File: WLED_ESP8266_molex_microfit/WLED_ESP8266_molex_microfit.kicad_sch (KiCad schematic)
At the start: 65 parts, among them J1 Molex Micro-fit 2x1, J2 Molex Micro-fit 3x1, J3 Molex Micro-fit 2x1, J4 Molex Micro-fit 2x1, J5 USB_B_Micro, J6 Molex Micro-fit 2x1, J7 Molex Micro-fit 3x1, J8 Molex Micro-fit 3x1, Q1 AO3401A, Q2 AO3401A, U1 ESP-12F, U2 TPS54331DDAR, U3 TXS0102DCT, U4 TXS0102DCT, U6 ME6211A33M3G-N

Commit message: Issue 28.01.Yannik_part1
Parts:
- R1, R10, R12, R13, R14, R15, R16, R17: footprint Capacitor_SMD:C_0402_1005Metric_Pad0.74x0.62mm_HandSolder -> Resistor_SMD:R_0402_1005Metric_Pad0.72x0.64mm_HandSolder
- R18, R7, R8, R9: footprint Capacitor_SMD:C_0603_1608Metric_Pad1.08x0.95mm_HandSolder -> Resistor_SMD:R_0603_1608Metric_Pad0.98x0.95mm_HandSolder
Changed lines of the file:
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@@
     (property "Reference" "R12" (id 0) (at 46.99 83.82 90))
     (property "Value" "10k" (id 1) (at 50.8 87.63 90))
-    (property "Footprint" "Capacitor_SMD:C_0402_1005Metric_Pad0.74x0.62mm_HandSolder" (id 2) (at 50.038 87.63 90)
+    (property "Footprint" "Resistor_SMD:R_0402_1005Metric_Pad0.72x0.64mm_HandSolder" (id 2) (at 50.038 87.63 90)
       (effects (font (size 1.27 1.27)) hide)
     )
@@
     (property "Reference" "R8" (id 0) (at 259.08 39.37 90))
     (property "Value" "300" (id 1) (at 255.27 43.18 90))
-    (property "Footprint" "Capacitor_SMD:C_0603_1608Metric_Pad1.08x0.95mm_HandSolder" (id 2) (at 255.27 42.418 90)
+    (property "Footprint" "Resistor_SMD:R_0603_1608Metric_Pad0.98x0.95mm_HandSolder" (id 2) (at 255.27 42.418 90)
       (effects (font (size 1.27 1.27)) hide)
     )
@@
     (property "Reference" "R17" (id 0) (at 166.37 91.44 90))
     (property "Value" "10k" (id 1) (at 171.45 92.71 90))
-    (property "Footprint" "Capacitor_SMD:C_0402_1005Metric_Pad0.74x0.62mm_HandSolder" (id 2) (at 170.688 92.71 90)
+    (property "Footprint" "Resistor_SMD:R_0402_1005Metric_Pad0.72x0.64mm_HandSolder" (id 2) (at 170.688 92.71 90)
       (effects (font (size 1.27 1.27)) hide)
     )
@@
     (property "Reference" "R15" (id 0) (at 118.11 91.44 90))
     (property "Value" "10k" (id 1) (at 123.19 92.71 90))
-    (property "Footprint" "Capacitor_SMD:C_0402_1005Metric_Pad0.74x0.62mm_HandSolder" (id 2) (at 122.428 92.71 90)
+    (property "Footprint" "Resistor_SMD:R_0402_1005Metric_Pad0.72x0.64mm_HandSolder" (id 2) (at 122.428 92.71 90)
       (effects (font (size 1.27 1.27)) hide)
     )
@@
     (property "Reference" "R9" (id 0) (at 259.08 90.17 90))
     (property "Value" "300" (id 1) (at 255.27 93.98 90))
-    (property "Footprint" "Capacitor_SMD:C_0603_1608Metric_Pad1.08x0.95mm_HandSolder" (id 2) (at 255.27 93.218 90)
+    (property "Footprint" "Resistor_SMD:R_0603_1608Metric_Pad0.98x0.95mm_HandSolder" (id 2) (at 255.27 93.218 90)
       (effects (font (size 1.27 1.27)) hide)
     )
@@
     (property "Reference" "R14" (id 0) (at 62.23 83.82 90))
     (property "Value" "10k" (id 1) (at 66.04 87.63 90))
-    (property "Footprint" "Capacitor_SMD:C_0402_1005Metric_Pad0.74x0.62mm_HandSolder" (id 2) (at 65.278 87.63 90)
+    (property "Footprint" "Resistor_SMD:R_0402_1005Metric_Pad0.72x0.64mm_HandSolder" (id 2) (at 65.278 87.63 90)
       (effects (font (size 1.27 1.27)) hide)
     )
@@
     (property "Reference" "R7" (id 0) (at 259.08 34.29 90))
     (property "Value" "300" (id 1) (at 255.27 38.1 90))
-    (property "Footprint" "Capacitor_SMD:C_0603_1608Metric_Pad1.08x0.95mm_HandSolder" (id 2) (at 255.27 37.338 90)
+    (property "Footprint" "Resistor_SMD:R_0603_1608Metric_Pad0.98x0.95mm_HandSolder" (id 2) (at 255.27 37.338 90)
       (effects (font (size 1.27 1.27)) hide)
     )
@@
     (property "Reference" "R1" (id 0) (at 17.78 86.36 90))
     (property "Value" "10k" (id 1) (at 21.59 90.17 90))
-    (property "Footprint" "Capacitor_SMD:C_0402_1005Metric_Pad0.74x0.62mm_HandSolder" (id 2) (at 20.828 90.17 90)
+    (property "Footprint" "Resistor_SMD:R_0402_1005Metric_Pad0.72x0.64mm_HandSolder" (id 2) (at 20.828 90.17 90)
       (effects (font (size 1.27 1.27)) hide)
     )
@@
     (property "Reference" "R16" (id 0) (at 158.75 26.67 90))
     (property "Value" "10k" (id 1) (at 162.56 30.48 90))
-    (property "Footprint" "Capacitor_SMD:C_0402_1005Metric_Pad0.74x0.62mm_HandSolder" (id 2) (at 161.798 30.48 90)
+    (property "Footprint" "Resistor_SMD:R_0402_1005Metric_Pad0.72x0.64mm_HandSolder" (id 2) (at 161.798 30.48 90)
       (effects (font (size 1.27 1.27)) hide)
     )
@@
     (property "Reference" "R10" (id 0) (at 267.97 63.5 90))
     (property "Value" "10k" (id 1) (at 273.05 63.5 90))
-    (property "Footprint" "Capacitor_SMD:C_0402_1005Metric_Pad0.74x0.62mm_HandSolder" (id 2) (at 272.288 63.5 90)
+    (property "Footprint" "Resistor_SMD:R_0402_1005Metric_Pad0.72x0.64mm_HandSolder" (id 2) (at 272.288 63.5 90)
       (effects (font (size 1.27 1.27)) hide)
     )
@@
     (property "Reference" "R18" (id 0) (at 205.74 133.35 90))
     (property "Value" "10k" (id 1) (at 209.55 137.16 90))
-    (property "Footprint" "Capacitor_SMD:C_0603_1608Metric_Pad1.08x0.95mm_HandSolder" (id 2) (at 208.788 137.16 90)
+    (property "Footprint" "Resistor_SMD:R_0603_1608Metric_Pad0.98x0.95mm_HandSolder" (id 2) (at 208.788 137.16 90)
       (effects (font (size 1.27 1.27)) hide)
     )
@@
     (property "Reference" "R13" (id 0) (at 54.61 83.82 90))
     (property "Value" "10k" (id 1) (at 58.42 87.63 90))
-    (property "Footprint" "Capacitor_SMD:C_0402_1005Metric_Pad0.74x0.62mm_HandSolder" (id 2) (at 57.658 87.63 90)
+    (property "Footprint" "Resistor_SMD:R_0402_1005Metric_Pad0.72x0.64mm_HandSolder" (id 2) (at 57.658 87.63 90)
       (effects (font (size 1.27 1.27)) hide)
     )
@@
     )
     (path "/d73f5447-4ae0-4c4a-a809-adb19f1201cd"
-      (reference "R1") (unit 1) (value "10k") (footprint "Capacitor_SMD:C_0402_1005Metric_Pad0.74x0.62mm_HandSolder")
+      (reference "R1") (unit 1) (value "10k") (footprint "Resistor_SMD:R_0402_1005Metric_Pad0.72x0.64mm_HandSolder")
     )
     (path "/9736f88a-f61b-412c-91c8-9d84934592a6"
@@
     )
     (path "/d25a3270-010c-46c6-957f-123f9bf187b7"
-      (reference "R7") (unit 1) (value "300") (footprint "Capacitor_SMD:C_0603_1608Metric_Pad1.08x0.95mm_HandSolder")
+      (reference "R7") (unit 1) (value "300") (footprint "Resistor_SMD:R_0603_1608Metric_Pad0.98x0.95mm_HandSolder")
     )
     (path "/41178f10-9942-424b-8ecb-9661f254316d"
-      (reference "R8") (unit 1) (value "300") (footprint "Capacitor_SMD:C_0603_1608Metric_Pad1.08x0.95mm_HandSolder")
+      (reference "R8") (unit 1) (value "300") (footprint "Resistor_SMD:R_0603_1608Metric_Pad0.98x0.95mm_HandSolder")
     )
     (path "/984f9213-4deb-4eff-b095-cde2ceafdd01"
-      (reference "R9") (unit 1) (value "300") (footprint "Capacitor_SMD:C_0603_1608Metric_Pad1.08x0.95mm_HandSolder")
+      (reference "R9") (unit 1) (value "300") (footprint "Resistor_SMD:R_0603_1608Metric_Pad0.98x0.95mm_HandSolder")
     )
     (path "/e21af3ac-6a90-40ab-8522-34cb00684b27"
-      (reference "R10") (unit 1) (value "10k") (footprint "Capacitor_SMD:C_0402_1005Metric_Pad0.74x0.62mm_HandSolder")
+      (reference "R10") (unit 1) (value "10k") (footprint "Resistor_SMD:R_0402_1005Metric_Pad0.72x0.64mm_HandSolder")
     )
     (path "/5aef3f3d-e3a1-42e7-aab5-b97ecd4f9ebd"
@@
     )
     (path "/0526c0f0-b604-4a5d-b668-a554f7870c57"
-      (reference "R12") (unit 1) (value "10k") (footprint "Capacitor_SMD:C_0402_1005Metric_Pad0.74x0.62mm_HandSolder")
+      (reference "R12") (unit 1) (value "10k") (footprint "Resistor_SMD:R_0402_1005Metric_Pad0.72x0.64mm_HandSolder")
     )
     (path "/f9fe30f9-fa00-46d5-a4e6-77d63a55d4b6"
-      (reference "R13") (unit 1) (value "10k") (footprint "Capacitor_SMD:C_0402_1005Metric_Pad0.74x0.62mm_HandSolder")
+      (reference "R13") (unit 1) (value "10k") (footprint "Resistor_SMD:R_0402_1005Metric_Pad0.72x0.64mm_HandSolder")
     )
     (path "/c462ec9b-ec5e-4e59-b306-0da8d6f70500"
-      (reference "R14") (unit 1) (value "10k") (footprint "Capacitor_SMD:C_0402_1005Metric_Pad0.74x0.62mm_HandSolder")
+      (reference "R14") (unit 1) (value "10k") (footprint "Resistor_SMD:R_0402_1005Metric_Pad0.72x0.64mm_HandSolder")
     )
     (path "/8bdcca36-89f8-4cc2-867e-e40b791a0029"
-      (reference "R15") (unit 1) (value "10k") (footprint "Capacitor_SMD:C_0402_1005Metric_Pad0.74x0.62mm_HandSolder")
+      (reference "R15") (unit 1) (value "10k") (footprint "Resistor_SMD:R_0402_1005Metric_Pad0.72x0.64mm_HandSolder")
     )
     (path "/d7a72f02-1984-4a3c-9afb-0ee7d0f20433"
-      (reference "R16") (unit 1) (value "10k") (footprint "Capacitor_SMD:C_0402_1005Metric_Pad0.74x0.62mm_HandSolder")
+      (reference "R16") (unit 1) (value "10k") (footprint "Resistor_SMD:R_0402_1005Metric_Pad0.72x0.64mm_HandSolder")
     )
     (path "/59799987-08dc-4288-9480-cfc9b65b7e76"
-      (reference "R17") (unit 1) (value "10k") (footprint "Capacitor_SMD:C_0402_1005Metric_Pad0.74x0.62mm_HandSolder")
+      (reference "R17") (unit 1) (value "10k") (footprint "Resistor_SMD:R_0402_1005Metric_Pad0.72x0.64mm_HandSolder")
     )
     (path "/f4a3769e-c888-4155-84d6-34953043327d"
-      (reference "R18") (unit 1) (value "10k") (footprint "Capacitor_SMD:C_0603_1608Metric_Pad1.08x0.95mm_HandSolder")
+      (reference "R18") (unit 1) (value "10k") (footprint "Resistor_SMD:R_0603_1608Metric_Pad0.98x0.95mm_HandSolder")
     )
     (path "/be1aa7ed-93c7-4da1-a65d-02d064f41f29"

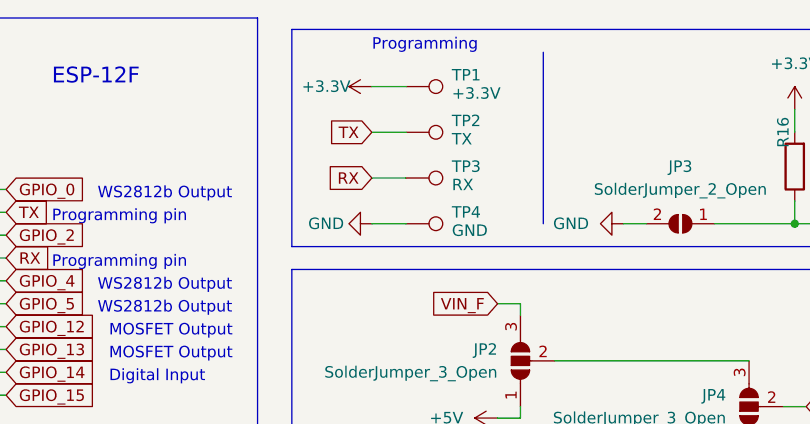
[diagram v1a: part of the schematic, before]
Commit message: feedback implemented
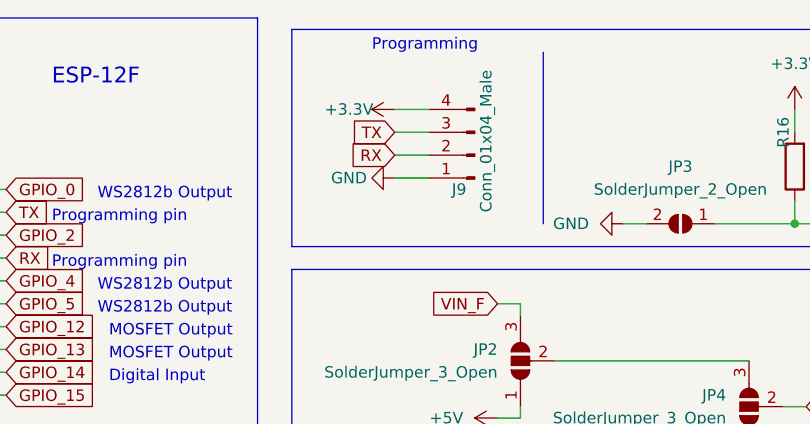
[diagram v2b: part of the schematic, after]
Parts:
- removed TP1: +3.3V, TestPoint:TestPoint_Pad_D1.5mm, symbol Connector:TestPoint
- removed TP2: TX, TestPoint:TestPoint_Pad_D1.5mm, symbol Connector:TestPoint
- removed TP3: RX, TestPoint:TestPoint_Pad_D1.5mm, symbol Connector:TestPoint
- removed TP4: GND, TestPoint:TestPoint_Pad_D1.5mm, symbol Connector:TestPoint
- added J9: Conn_01x04_Male, Connector_PinHeader_2.54mm:PinHeader_1x04_P2.54mm_Vertical, symbol Connector:Conn_01x04_Male
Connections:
- net +3V3: now also J9.4 (Pin_4)
- net GND: now also J9.1 (Pin_1)
- net RX: now also J9.2 (Pin_2)
- net TX: now also J9.3 (Pin_3)
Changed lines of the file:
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@@
     (stroke (width 0) (type default) (color 0 0 0 0))
   )
-  (wire (pts (xy 113.03 26.67) (xy 116.84 26.67))
+  (wire (pts (xy 115.57 26.67) (xy 119.38 26.67))
     (stroke (width 0) (type default) (color 0 0 0 0))
   )
@@
     (stroke (width 0) (type default) (color 0 0 0 0))
   )
-  (wire (pts (xy 113.03 36.83) (xy 116.84 36.83))
+  (wire (pts (xy 115.57 31.75) (xy 119.38 31.75))
     (stroke (width 0) (type default) (color 0 0 0 0))
   )
@@
     (stroke (width 0) (type default) (color 0 0 0 0))
   )
-  (wire (pts (xy 113.03 21.59) (xy 116.84 21.59))
+  (wire (pts (xy 115.57 24.13) (xy 119.38 24.13))
     (stroke (width 0) (type default) (color 0 0 0 0))
   )
@@
     (stroke (width 0) (type default) (color 0 0 0 0))
   )
-  (wire (pts (xy 113.03 31.75) (xy 116.84 31.75))
+  (wire (pts (xy 115.57 29.21) (xy 119.38 29.21))
     (stroke (width 0) (type default) (color 0 0 0 0))
   )
@@
     )
   )
-  (global_label "RX" (shape input) (at 113.03 31.75 180) (fields_autoplaced)
+  (global_label "RX" (shape input) (at 115.57 29.21 180) (fields_autoplaced)
     (effects (font (size 1.27 1.27)) (justify right))
-    (property "Intersheet References" "${INTERSHEET_REFS}" (id 0) (at 108.1374 31.6706 0)
+    (property "Intersheet References" "${INTERSHEET_REFS}" (id 0) (at 110.6774 29.1306 0)
       (effects (font (size 1.27 1.27)) (justify right) hide)
     )
@@
     )
   )
-  (global_label "TX" (shape input) (at 113.03 26.67 180) (fields_autoplaced)
+  (global_label "TX" (shape input) (at 115.57 26.67 180) (fields_autoplaced)
     (effects (font (size 1.27 1.27)) (justify right))
-    (property "Intersheet References" "${INTERSHEET_REFS}" (id 0) (at 108.4398 26.5906 0)
+    (property "Intersheet References" "${INTERSHEET_REFS}" (id 0) (at 110.9798 26.5906 0)
       (effects (font (size 1.27 1.27)) (justify right) hide)
     )
@@
     (pin "1")
   )
-  (symbol (lib_id "power:GND") (at 113.03 36.83 270) (unit 1)
+  (symbol (lib_id "power:GND") (at 115.57 31.75 270) (unit 1)
     (in_bom yes) (on_board yes)
-    (property "Reference" "#PWR0146" (id 0) (at 106.68 36.83 0)
+    (property "Reference" "#PWR0146" (id 0) (at 109.22 31.75 0)
       (effects (font (size 1.27 1.27)) hide)
     )
-    (property "Value" "GND" (id 1) (at 107.95 36.83 90))
-    (property "Footprint" "" (id 2) (at 113.03 36.83 0)
+    (property "Value" "GND" (id 1) (at 110.49 31.75 90))
+    (property "Footprint" "" (id 2) (at 115.57 31.75 0)
       (effects (font (size 1.27 1.27)) hide)
     )
-    (property "Datasheet" "" (id 3) (at 113.03 36.83 0)
+    (property "Datasheet" "" (id 3) (at 115.57 31.75 0)
       (effects (font (size 1.27 1.27)) hide)
     )
@@
     (pin "1")
   )
-  (symbol (lib_id "power:+3.3V") (at 113.03 21.59 90) (unit 1)
+  (symbol (lib_id "power:+3.3V") (at 115.57 24.13 90) (unit 1)
     (in_bom yes) (on_board yes)
-    (property "Reference" "#PWR0145" (id 0) (at 116.84 21.59 0)
+    (property "Reference" "#PWR0145" (id 0) (at 119.38 24.13 0)
       (effects (font (size 1.27 1.27)) hide)
     )
-    (property "Value" "+3.3V" (id 1) (at 107.95 21.59 90))
-    (property "Footprint" "" (id 2) (at 113.03 21.59 0)
+    (property "Value" "+3.3V" (id 1) (at 110.49 24.13 90))
+    (property "Footprint" "" (id 2) (at 115.57 24.13 0)
       (effects (font (size 1.27 1.27)) hide)
     )
-    (property "Datasheet" "" (id 3) (at 113.03 21.59 0)
+    (property "Datasheet" "" (id 3) (at 115.57 24.13 0)
       (effects (font (size 1.27 1.27)) hide)
     )
@@
     (pin "1")
   )
-  (symbol (lib_id "Connector:TestPoint") (at 116.84 21.59 270) (unit 1)
-    (in_bom yes) (on_board yes)
-    (property "Reference" "TP1" (id 0) (at 121.92 20.32 90)
-      (effects (font (size 1.27 1.27)) (justify left))
-    )
-    (property "Value" "+3.3V" (id 1) (at 121.92 22.3521 90)
-      (effects (font (size 1.27 1.27)) (justify left))
-    )
-    (property "Footprint" "TestPoint:TestPoint_Pad_D1.5mm" (id 2) (at 116.84 26.67 0)
-      (effects (font (size 1.27 1.27)) hide)
-    )
-    (property "Datasheet" "~" (id 3) (at 116.84 26.67 0)
-      (effects (font (size 1.27 1.27)) hide)
-    )
-    (pin "1")
-  )
   (symbol (lib_id "Regulator_Linear:AMS1117CD-3.3") (at 129.54 121.92 0) (unit 1)
     (in_bom yes) (on_board yes) (fields_autoplaced)
@@
     (pin "1")
   )
-  (symbol (lib_id "Connector:TestPoint") (at 116.84 31.75 270) (unit 1)
-    (in_bom yes) (on_board yes)
-    (property "Reference" "TP3" (id 0) (at 121.92 30.48 90)
-      (effects (font (size 1.27 1.27)) (justify left))
-    )
-    (property "Value" "RX" (id 1) (at 121.92 32.5121 90)
-      (effects (font (size 1.27 1.27)) (justify left))
-    )
-    (property "Footprint" "TestPoint:TestPoint_Pad_D1.5mm" (id 2) (at 116.84 36.83 0)
-      (effects (font (size 1.27 1.27)) hide)
-    )
-    (property "Datasheet" "~" (id 3) (at 116.84 36.83 0)
-      (effects (font (size 1.27 1.27)) hide)
-    )
-    (pin "1")
-  )
   (symbol (lib_id "power:GND") (at 251.46 138.43 270) (unit 1)
     (in_bom yes) (on_board yes) (fields_autoplaced)
@@
     (pin "3")
   )
-  (symbol (lib_id "Connector:TestPoint") (at 116.84 26.67 270) (unit 1)
-    (in_bom yes) (on_board yes)
-    (property "Reference" "TP2" (id 0) (at 121.92 25.4 90)
-      (effects (font (size 1.27 1.27)) (justify left))
-    )
-    (property "Value" "TX" (id 1) (at 121.92 27.4321 90)
-      (effects (font (size 1.27 1.27)) (justify left))
-    )
-    (property "Footprint" "TestPoint:TestPoint_Pad_D1.5mm" (id 2) (at 116.84 31.75 0)
-      (effects (font (size 1.27 1.27)) hide)
-    )
-    (property "Datasheet" "~" (id 3) (at 116.84 31.75 0)
-      (effects (font (size 1.27 1.27)) hide)
-    )
-    (pin "1")
-  )
   (symbol (lib_id "Device:C") (at 231.14 22.86 90) (unit 1)
     (in_bom yes) (on_board yes)
@@
     (pin "1")
   )
-  (symbol (lib_id "Connector:TestPoint") (at 116.84 36.83 270) (unit 1)
-    (in_bom yes) (on_board yes)
-    (property "Reference" "TP4" (id 0) (at 121.92 35.56 90)
-      (effects (font (size 1.27 1.27)) (justify left))
-    )
-    (property "Value" "GND" (id 1) (at 121.92 37.5921 90)
-      (effects (font (size 1.27 1.27)) (justify left))
-    )
-    (property "Footprint" "TestPoint:TestPoint_Pad_D1.5mm" (id 2) (at 116.84 41.91 0)
-      (effects (font (size 1.27 1.27)) hide)
-    )
-    (property "Datasheet" "~" (id 3) (at 116.84 41.91 0)
-      (effects (font (size 1.27 1.27)) hide)
-    )
-    (pin "1")
-  )
   (symbol (lib_id "Device:R") (at 270.51 63.5 180) (unit 1)
     (in_bom yes) (on_board yes)
@@
     (pin "2")
   )
+  (symbol (lib_id "Connector:Conn_01x04_Male") (at 124.46 29.21 180) (unit 1)
+    (in_bom yes) (on_board yes)
+    (property "Reference" "J9" (id 0) (at 121.92 33.02 0)
+      (effects (font (size 1.27 1.27)) (justify right))
+    )
+    (property "Value" "Conn_01x04_Male" (id 1) (at 125.73 35.56 90)
+      (effects (font (size 1.27 1.27)) (justify right))
+    )
+    (property "Footprint" "Connector_PinHeader_2.54mm:PinHeader_1x04_P2.54mm_Vertical" (id 2) (at 124.46 29.21 0)
+      (effects (font (size 1.27 1.27)) hide)
+    )
+    (property "Datasheet" "~" (id 3) (at 124.46 29.21 0)
+      (effects (font (size 1.27 1.27)) hide)
+    )
+    (pin "1")
+    (pin "2")
+    (pin "3")
+    (pin "4")
+  )
   (symbol (lib_id "Device:R") (at 55.88 87.63 180) (unit 1)
     (in_bom yes) (on_board yes)
@@
       (reference "J8") (unit 1) (value "Molex Micro-fit 3x1") (footprint "Connector_Molex:Molex_Micro-Fit_3.0_43650-0300_1x03_P3.00mm_Horizontal")
     )
+    (path "/f901e912-c299-49a9-b1d9-f9b63f35df46"
+      (reference "J9") (unit 1) (value "Conn_01x04_Male") (footprint "Connector_PinHeader_2.54mm:PinHeader_1x04_P2.54mm_Vertical")
+    )
     (path "/f14a0100-bc3e-4b3a-b1ca-db976ded308e"
       (reference "JP1") (unit 1) (value "SolderJumper_2_Open") (footprint "Jumper:SolderJumper-2_P1.3mm_Open_RoundedPad1.0x1.5mm")
@@
       (reference "R19") (unit 1) (value "1M") (footprint "Resistor_SMD:R_0805_2012Metric")
     )
-    (path "/63405878-cf3b-44a2-abdf-7ac907f9453d"
-      (reference "TP1") (unit 1) (value "+3.3V") (footprint "TestPoint:TestPoint_Pad_D1.5mm")
-    )
-    (path "/ab4c9366-637c-43ce-8605-21e0d4b4a7a7"
-      (reference "TP2") (unit 1) (value "TX") (footprint "TestPoint:TestPoint_Pad_D1.5mm")
-    )
-    (path "/9af74590-7b7f-4864-b1de-2868af720204"
-      (reference "TP3") (unit 1) (value "RX") (footprint "TestPoint:TestPoint_Pad_D1.5mm")
-    )
-    (path "/e0cbf46e-8228-4b92-be43-92541b68ac5e"
-      (reference "TP4") (unit 1) (value "GND") (footprint "TestPoint:TestPoint_Pad_D1.5mm")
-    )
     (path "/6f61acf9-283e-43c1-b11a-174e497e5b25"
